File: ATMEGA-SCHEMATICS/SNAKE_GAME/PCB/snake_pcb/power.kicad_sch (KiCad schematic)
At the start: 9 parts, among them J4 Barrel_Jack_Switch, U9 AMS1117-3.3

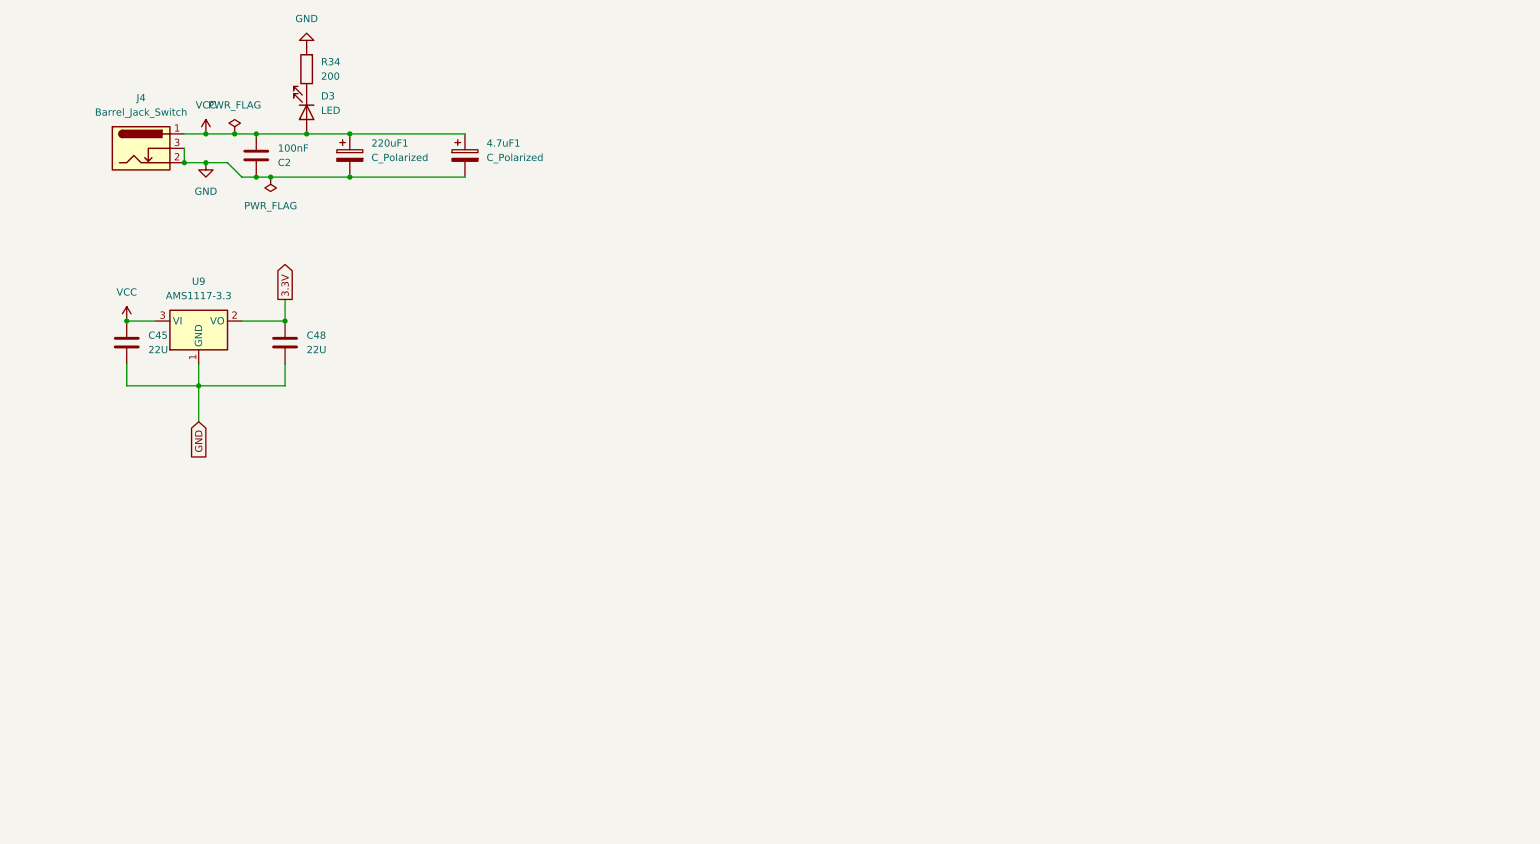
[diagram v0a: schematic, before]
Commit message: .
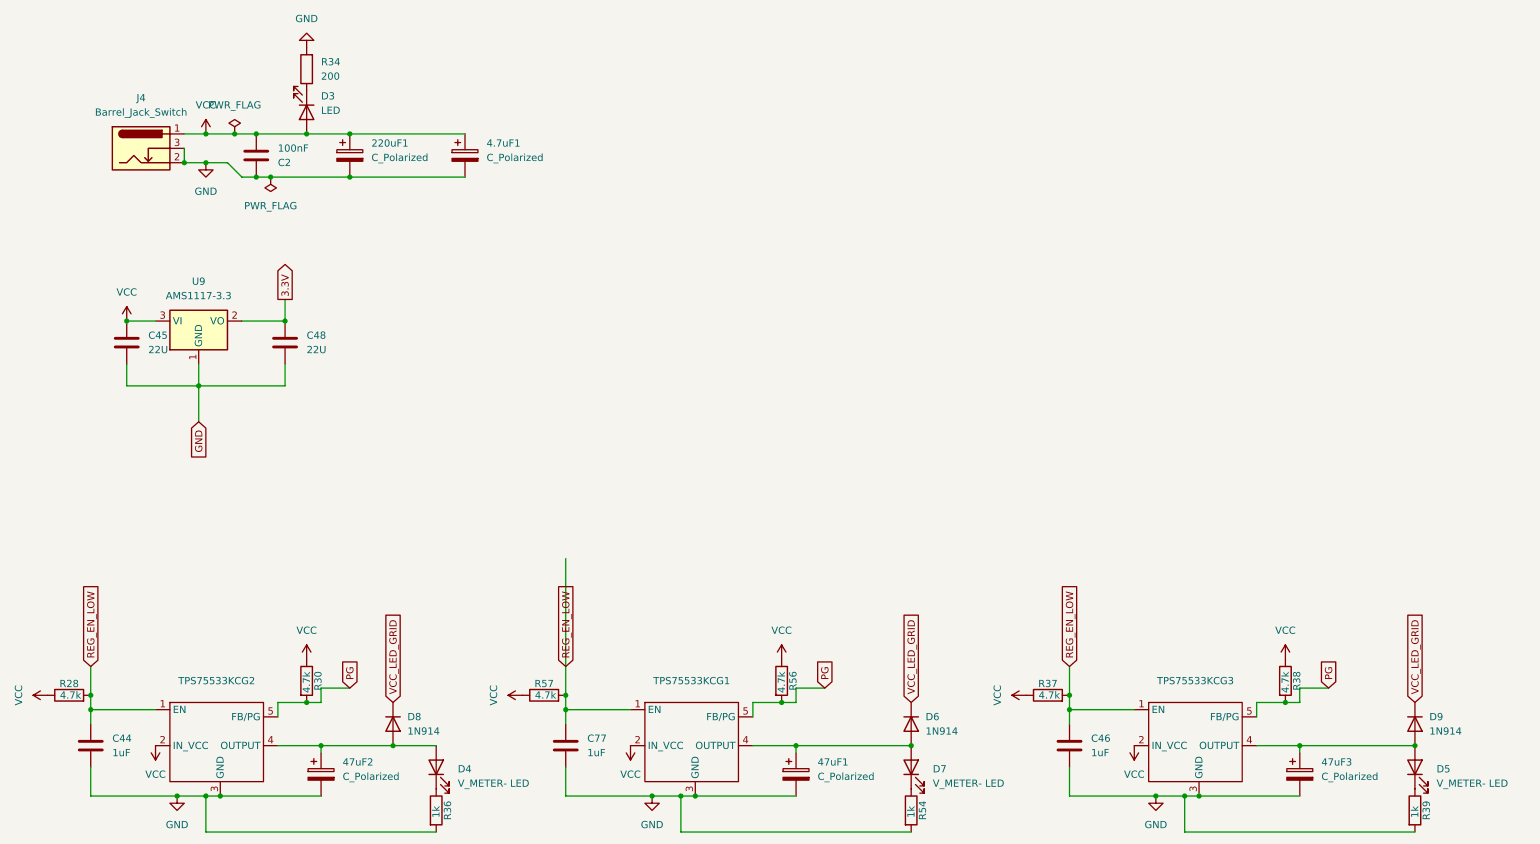
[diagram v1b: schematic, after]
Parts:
- added 47uF1, 47uF2, 47uF3: C_Polarized, Capacitor_THT:C_Disc_D3.0mm_W1.6mm_P2.50mm, symbol Device:C_Polarized
- added C44, C46, C77: 1uF, Capacitor_THT:C_Disc_D7.5mm_W5.0mm_P5.00mm, symbol Device:C
- added D4, D5, D7: V_METER- LED, LED_THT:LED_D1.8mm_W3.3mm_H2.4mm, symbol Device:LED
- added D6, D8, D9: 1N914, Diode_THT:D_DO-35_SOD27_P7.62mm_Horizontal, symbol Diode:1N914
- added R28, R30, R37, R38, R56, R57: 4.7k, Resistor_THT:R_Axial_DIN0207_L6.3mm_D2.5mm_P10.16mm_Horizontal, symbol Device:R
- added R36, R39, R54: 1k, Resistor_THT:R_Axial_DIN0207_L6.3mm_D2.5mm_P10.16mm_Horizontal, symbol Device:R
- added TPS75533KCG1, TPS75533KCG2, TPS75533KCG3: ~, Package_TO_SOT_THT:TO-220-5_Vertical, symbol lucasLib:TPS75533KCG3
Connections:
- net GND: now also 47uF1.2, 47uF2.2, 47uF3.2, C44.2, C46.2, C77.2, R36.2, R39.2, R54.2, TPS75533KCG1.3 (GND), TPS75533KCG2.3 (GND), TPS75533KCG3.3 (GND)
- net VCC: now also R28.1, R30.1, R37.1, R38.1, R56.1, R57.1, TPS75533KCG1.2 (IN_VCC), TPS75533KCG2.2 (IN_VCC), TPS75533KCG3.2 (IN_VCC)
- new net: D7.1 (K), R54.1
- new net: 47uF1.1, D6.2 (A), D7.2 (A), TPS75533KCG1.4 (OUTPUT)
- new net: D4.1 (K), R36.1
- new net: 47uF2.1, D4.2 (A), D8.2 (A), TPS75533KCG2.4 (OUTPUT)
- new net: 47uF3.1, D5.2 (A), D9.2 (A), TPS75533KCG3.4 (OUTPUT)
- new net: D5.1 (K), R39.1
- new net PG: R30.2, R38.2, R56.2, TPS75533KCG1.5 (FB/PG), TPS75533KCG2.5 (FB/PG), TPS75533KCG3.5 (FB/PG)
- new net REG_EN_LOW: C44.1, C46.1, C77.1, R28.2, R37.2, R57.2, TPS75533KCG1.1 (EN), TPS75533KCG2.1 (EN), TPS75533KCG3.1 (EN)
- new net VCC_LED_GRID: D6.1 (K), D8.1 (K), D9.1 (K)
